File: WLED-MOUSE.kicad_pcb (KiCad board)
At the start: 4 copper layers, 54.4 x 67.6 mm, 20 parts, among them J1 FTDI-header, J2 Power-in, J4 Pixel-strip, J6 Pixel-strip, J7 Pixel-strip, J8 Pixel-strip, M1 INMP441, M2 INMP441-TH, SW1 SW_MEC_5E, SW2 SW_MEC_5E, U1 ESP32-WROOM-32D, U2 ESP32-WROOM-32D, U3 SN74LV4T125

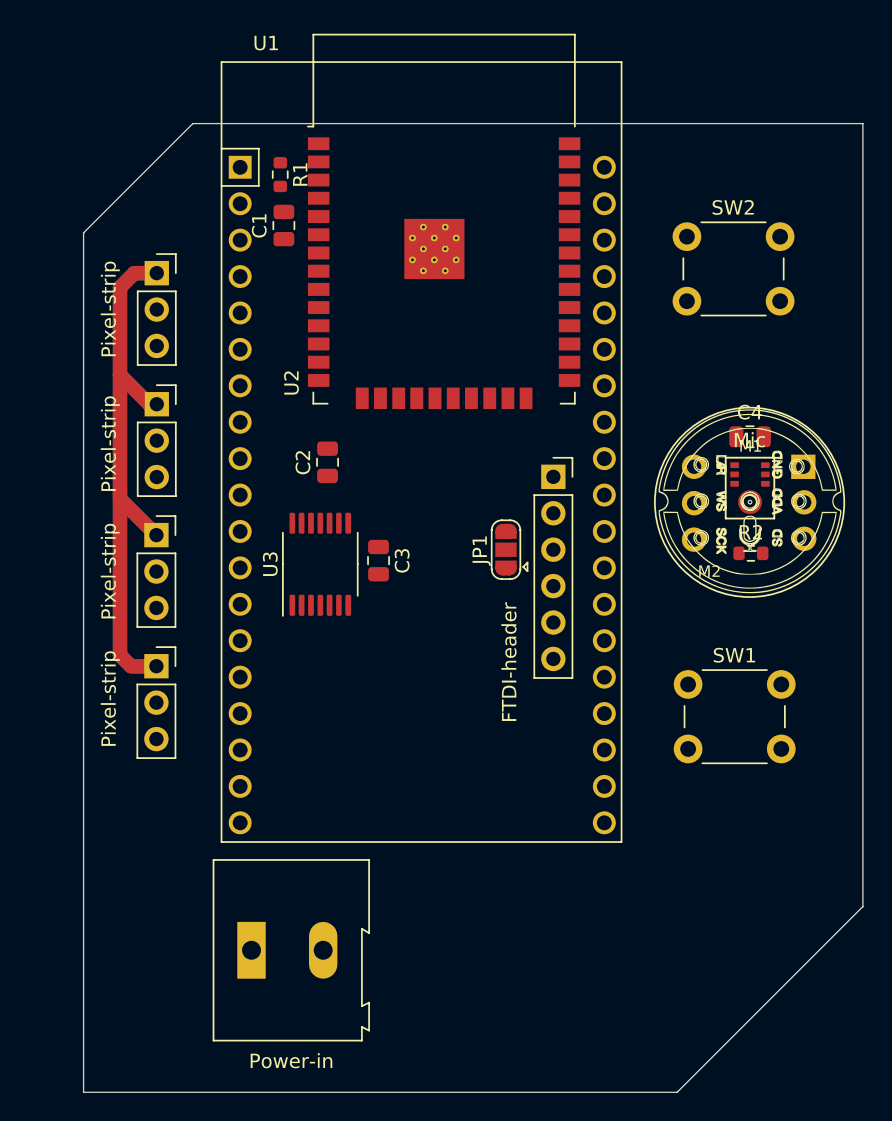
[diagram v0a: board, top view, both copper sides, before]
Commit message: started some routing and layout stuff
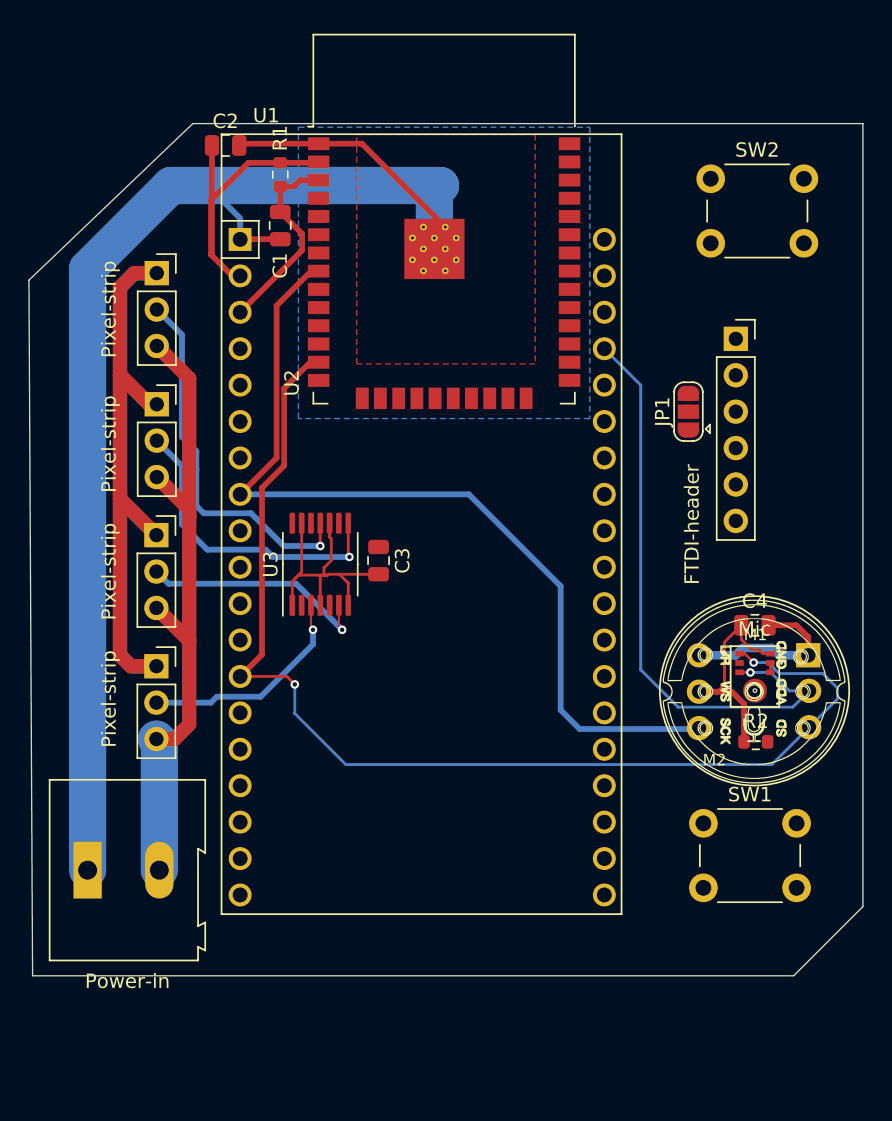
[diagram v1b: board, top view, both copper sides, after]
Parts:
- moved C2 23.2 mm to (167.1, 81.3), turned to 0 degrees
- moved J1 16.0 mm to (202.7, 94.8)
- moved JP1 16.0 mm to (199.4, 99.8)
- moved R2 13.2 mm to (204.1, 122.9)
- moved C4 13.2 mm to (204.1, 114.7)
- moved M1 13.2 mm to (204.1, 118.3)
- moved M2 13.2 mm to (204.0, 119.3)
- moved J2 12.7 mm to (157.5, 131.8)
- moved SW1 9.75 mm to (200.5, 128.6)
- moved U1 5.03 mm to (168.1, 87.8)
- moved SW2 4.37 mm to (201.0, 83.6)
- moved C1 0.25 mm to (170.9, 86.9), turned to -90 degrees
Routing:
- net GND: track 0.00 -> 132.4 mm
- net /SCK: track 0.00 -> 80.4 mm, vias 0 -> 2
- net /SD: track 0.00 -> 62.0 mm
- net +5V: track 0.00 -> 46.2 mm
- net /WS: track 0.00 -> 42.1 mm, vias 0 -> 1
- net +3.3V: track 0.00 -> 37.6 mm
- net Net-(J8-Pad2): track 0.00 -> 26.2 mm, vias 0 -> 1
- net Net-(J7-Pad2): track 0.00 -> 21.6 mm, vias 0 -> 1
- net Net-(J6-Pad2): track 0.00 -> 16.4 mm, vias 0 -> 1
- net Net-(J4-Pad2): track 0.00 -> 15.4 mm, vias 0 -> 1
- net /Reset: track 0.00 -> 14.1 mm
- added copper zone on B.Cu, net GND
- added copper zone on F.Cu, net GND
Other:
- board size 54.4 x 67.6 mm -> 58.2 x 59.4 mm
